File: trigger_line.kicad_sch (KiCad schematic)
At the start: 20 parts, among them P1 53048-0910, P2 53048-1010, U1 ILQ30, U2 ILQ30

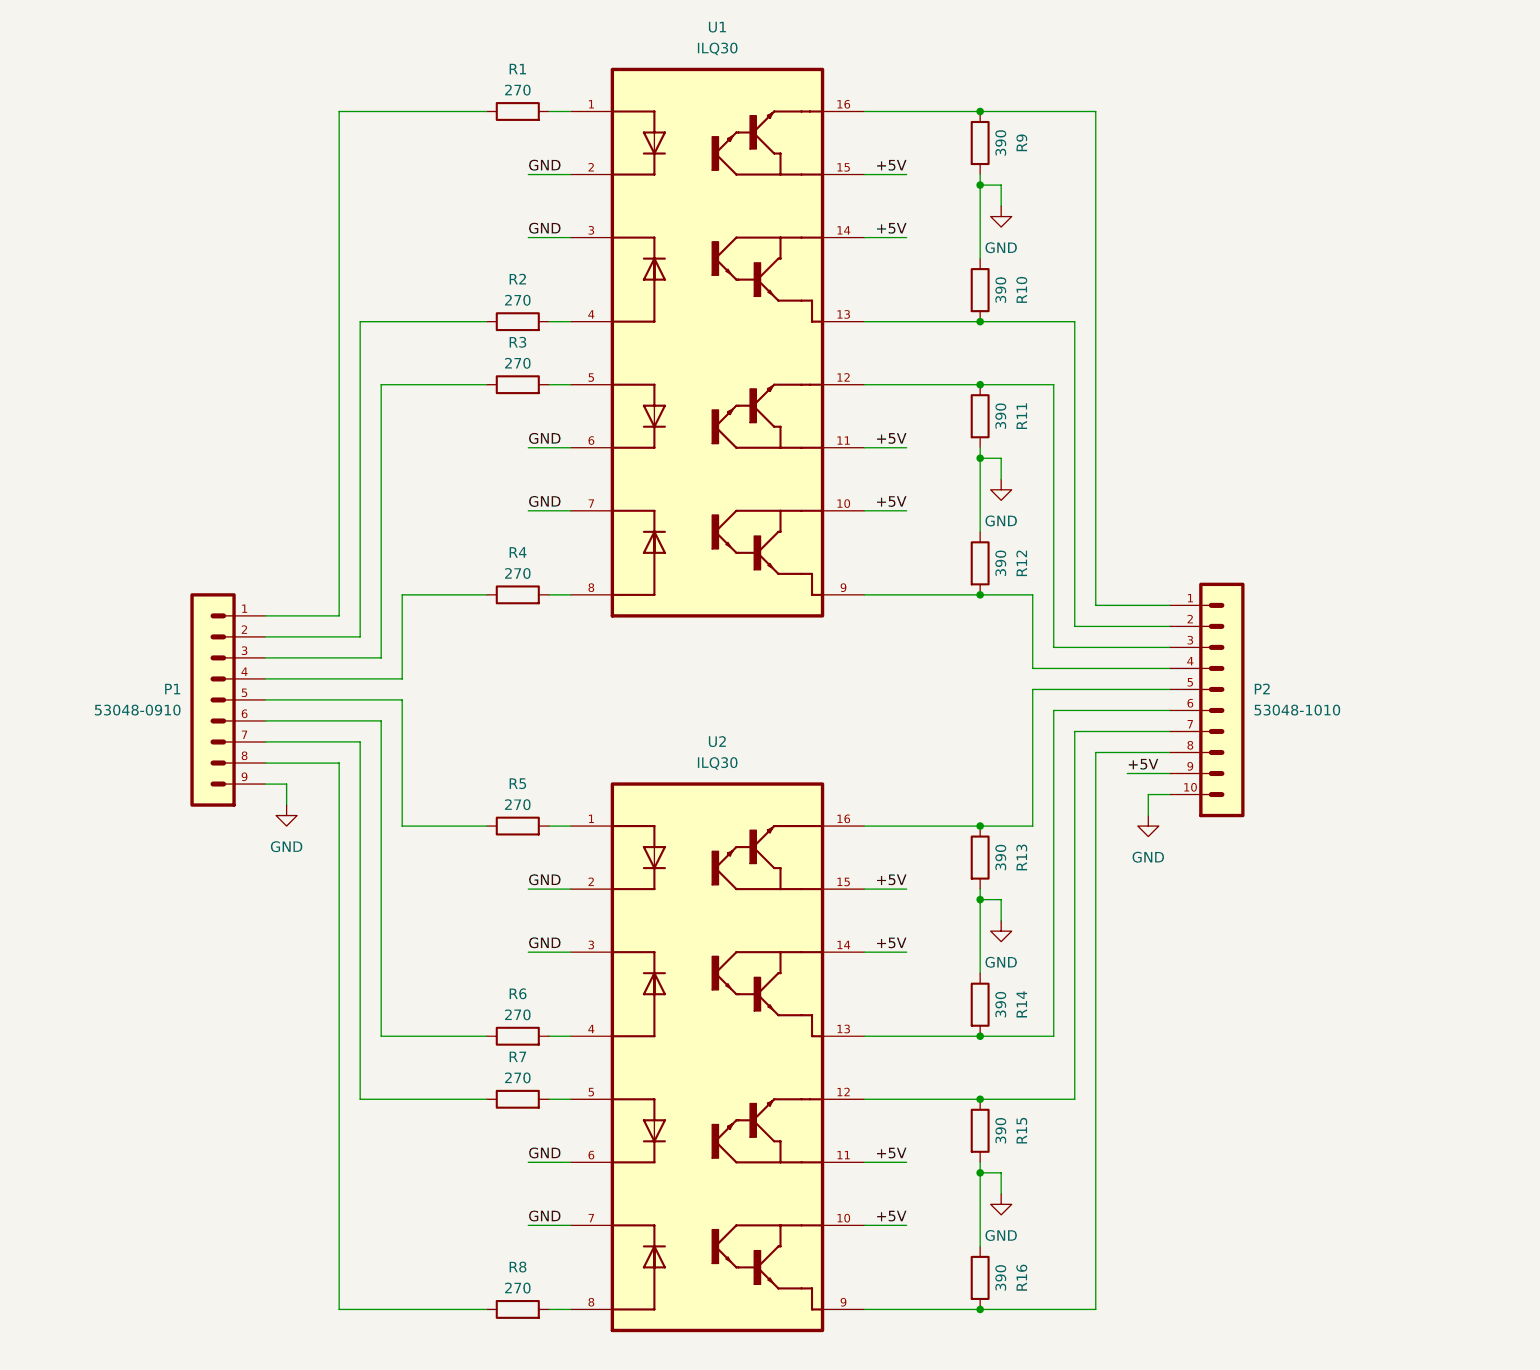
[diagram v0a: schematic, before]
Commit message: first order
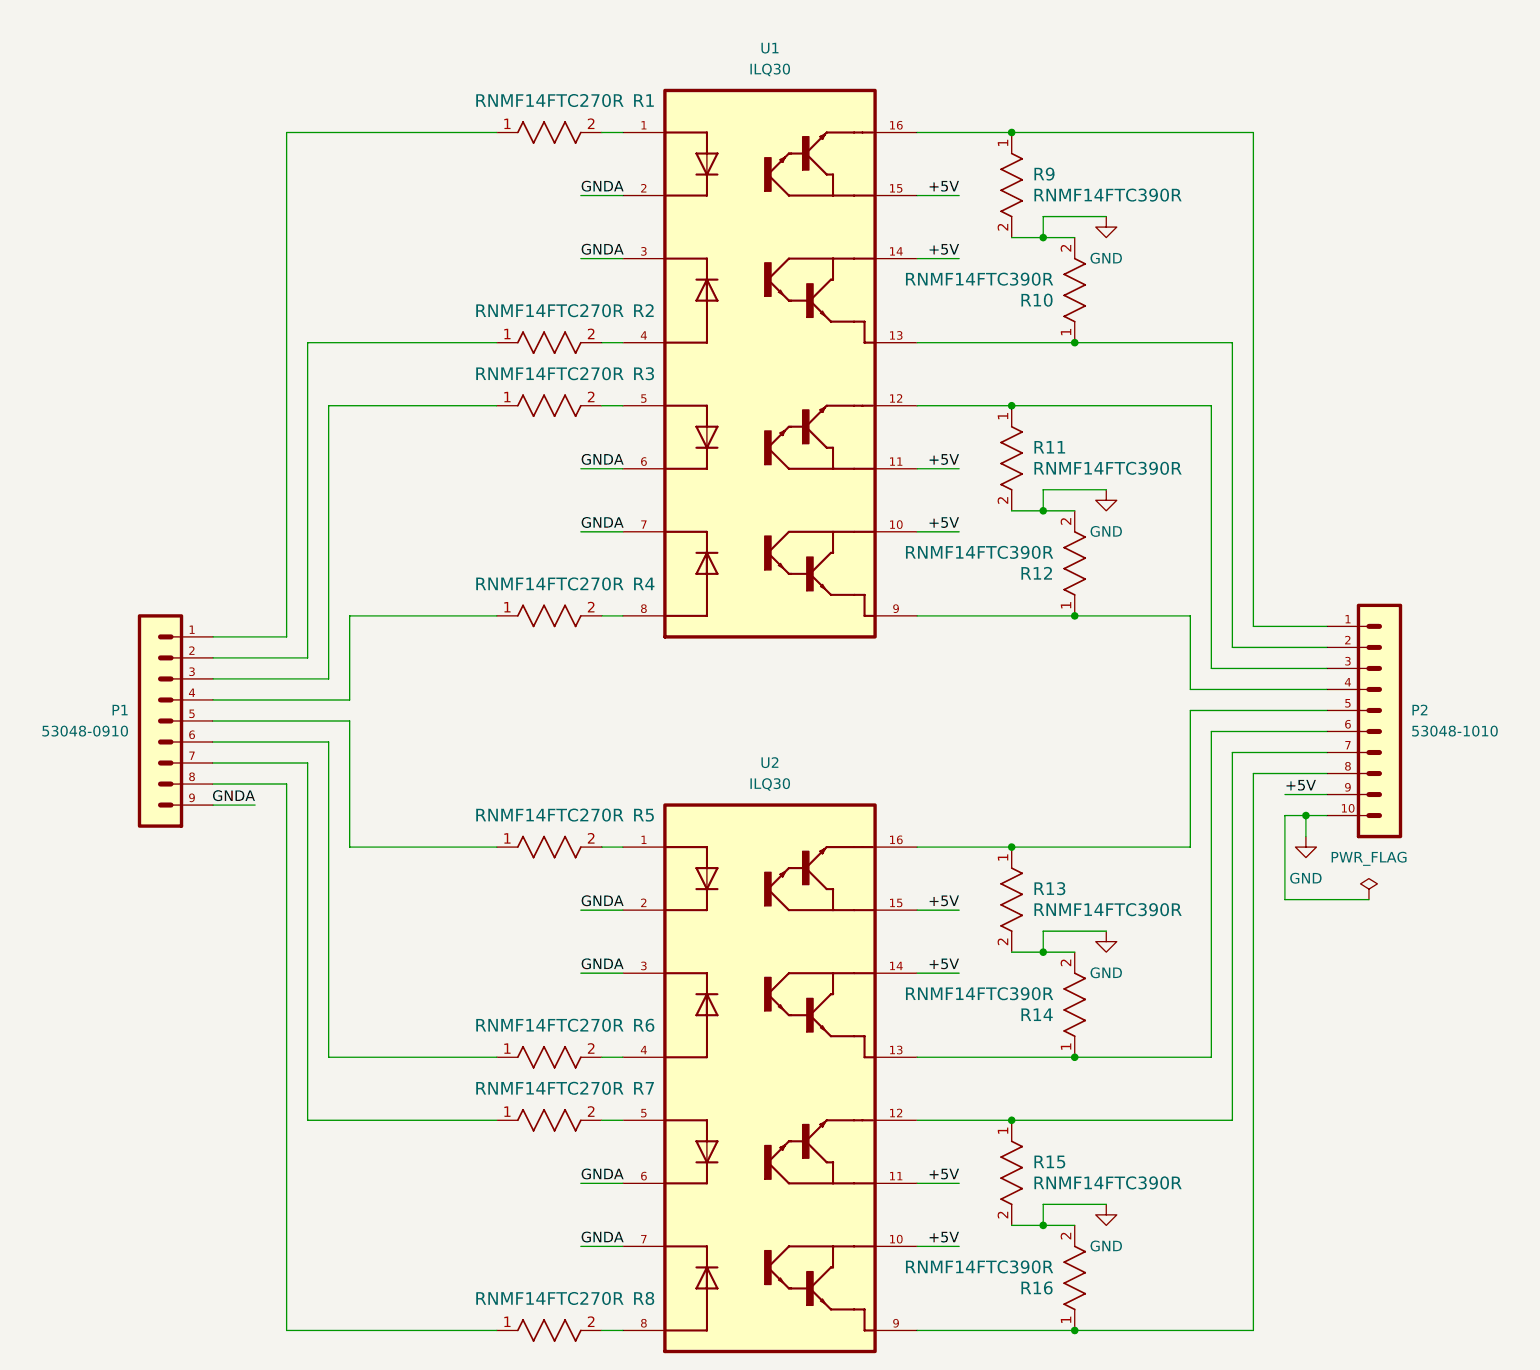
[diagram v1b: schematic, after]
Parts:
- removed R1, R2, R3, R4, R5, R6, R7, R8: 270, symbol Device:R
- removed R10, R11, R12, R13, R14, R15, R16, R9: 390, symbol Device:R
- added R1, R2, R3, R4, R5, R6, R7, R8: RNMF14FTC270R, STA_RNMF14_STP, symbol 2024-01-01_18-12-41:RNMF14FTC270R
- added R10, R11, R12, R13, R14, R15, R16, R9: RNMF14FTC390R, STA_RNMF14_STP, symbol 2024-01-01_18-12-10:RNMF14FTC390R
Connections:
- net GND: now also R10.2, R11.2, R12.2, R13.2, R14.2, R15.2, R16.2, R9.2; no longer P1.9, U1.2, U1.3, U1.6, U1.7, U2.2, U2.3, U2.6, U2.7
- net at P1.3: now also R3.1
- net at U1.5: now also R3.2
- net at P2.8, U2.9: now also R16.1
- net at U2.1: now also R5.2
- net at P2.7, U2.12: now also R15.1
- net at P2.6, U2.13: now also R14.1
- net at P2.5, U2.16: now also R13.1
- net at U2.4: now also R6.2
- net at U2.5: now also R7.2
- net at U2.8: now also R8.2
- net at P2.1, U1.16: now also R9.1
- net at P2.2, U1.13: now also R10.1
- net at P2.3, U1.12: now also R11.1
- net at P2.4, U1.9: now also R12.1
- net at U1.1: now also R1.2
- net at U1.4: now also R2.2
- net at U1.8: now also R4.2
- net at P1.6: now also R6.1
- net at P1.1: now also R1.1
- net at P1.2: now also R2.1
- net at P1.4: now also R4.1
- net at P1.5: now also R5.1
- net at P1.7: now also R7.1
- net at P1.8: now also R8.1
- new net GNDA: P1.9, U1.2, U1.3, U1.6, U1.7, U2.2, U2.3, U2.6, U2.7
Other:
- moved on the sheet: P1, P2, U1, U2
